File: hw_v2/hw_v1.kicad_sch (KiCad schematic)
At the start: 55 parts, among them J16 47352-1001, J8 USB_B, J9 Tag connect, SW2 SW_Push, U13 STM32F407VGTx, U14 TJA1051T-3, U15 25Q16, U16 REF3033, U17 SRV05-4, Y1 32.768kHz, Y2 25MHz

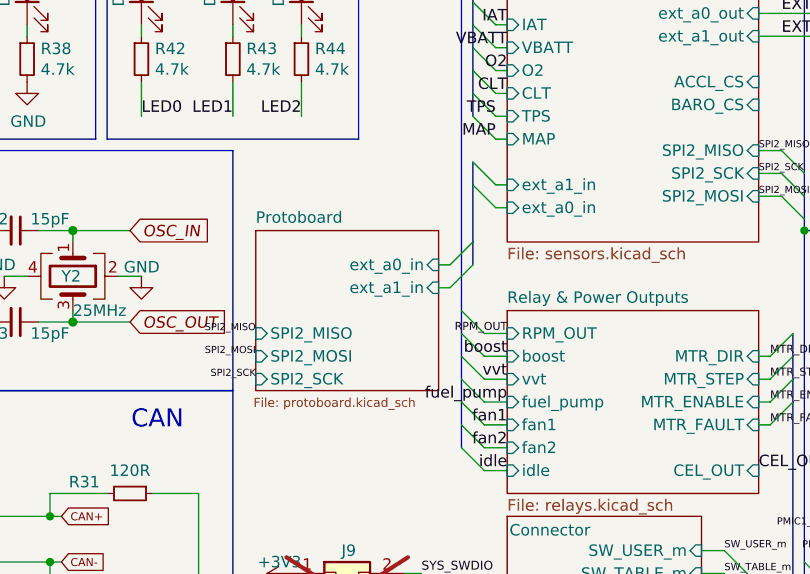
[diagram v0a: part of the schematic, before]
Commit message: wip v7
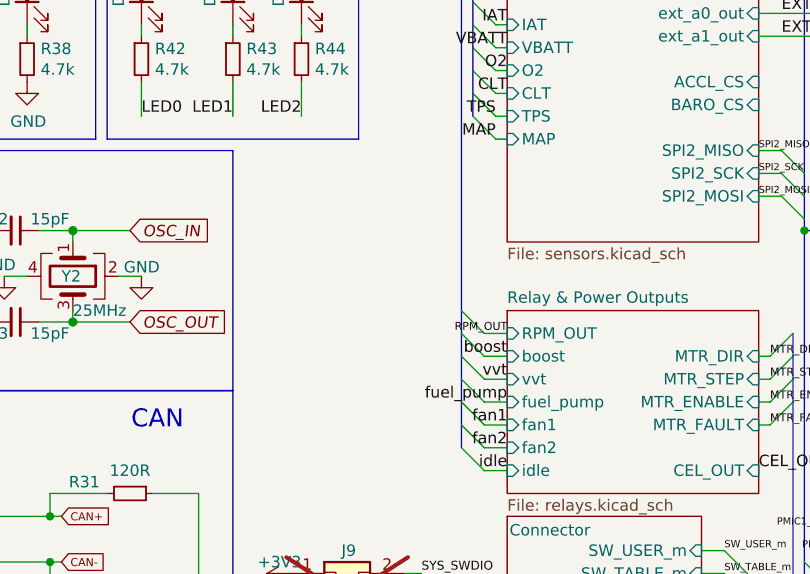
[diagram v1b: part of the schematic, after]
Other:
- removed sheet Protoboard
- sheet Sensors ports: added none; removed ext_a0_in, ext_a1_in
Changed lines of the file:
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@@
 	)
 	(bus_entry
-		(at 199.39 116.84)
-		(size 2.54 -2.54)
-		(stroke
-			(width 0)
-			(type default)
-		)
-	)
-	(bus_entry
 		(at 278.13 91.44)
 		(size 2.54 -2.54)
@@
 	)
 	(bus_entry
-		(at 201.93 105.41)
-		(size 2.54 2.54)
-		(stroke
-			(width 0)
-			(type default)
-		)
-	)
-	(bus_entry
 		(at 201.93 87.63)
 		(size 2.54 2.54)
@@
 	)
 	(bus_entry
-		(at 201.93 102.87)
-		(size 2.54 2.54)
-		(stroke
-			(width 0)
-			(type default)
-		)
-	)
-	(bus_entry
 		(at 88.9 66.04)
 		(size 2.54 2.54)
@@
 	)
 	(bus_entry
-		(at 199.39 114.3)
-		(size 2.54 -2.54)
-		(stroke
-			(width 0)
-			(type default)
-		)
-	)
-	(bus_entry
 		(at 276.86 154.94)
 		(size 2.54 -2.54)
@@
 	(wire
 		(pts
-			(xy 204.47 105.41) (xy 205.74 105.41)
-		)
-		(stroke
-			(width 0)
-			(type default)
-		)
-	)
-	(wire
-		(pts
 			(xy 81.28 124.46) (xy 95.25 124.46)
 		)
@@
 		)
 	)
-	(bus
-		(pts
-			(xy 201.93 102.87) (xy 201.93 105.41)
-		)
-		(stroke
-			(width 0)
-			(type default)
-		)
-	)
 	(wire
 		(pts
@@
 	(wire
 		(pts
-			(xy 198.12 116.84) (xy 199.39 116.84)
-		)
-		(stroke
-			(width 0)
-			(type default)
-		)
-	)
-	(wire
-		(pts
 			(xy 161.29 139.7) (xy 154.94 139.7)
 		)
@@
 		)
 	)
-	(wire
-		(pts
-			(xy 204.47 107.95) (xy 205.74 107.95)
-		)
-		(stroke
-			(width 0)
-			(type default)
-		)
-	)
 	(bus
 		(pts
@@
 	(wire
 		(pts
-			(xy 198.12 114.3) (xy 199.39 114.3)
-		)
-		(stroke
-			(width 0)
-			(type default)
-		)
-	)
-	(wire
-		(pts
 			(xy 55.88 38.1) (xy 55.88 40.64)
 		)
@@
 		)
 	)
-	(bus
-		(pts
-			(xy 201.93 111.76) (xy 201.93 114.3)
-		)
-		(stroke
-			(width 0)
-			(type default)
-		)
-	)
 	(wire
 		(pts
@@
 		)
 	)
-	(bus
-		(pts
-			(xy 201.93 105.41) (xy 201.93 111.76)
-		)
-		(stroke
-			(width 0)
-			(type default)
-		)
-	)
 	(wire
 		(pts
@@
 	)
 	(label "SPI2_MOSI"
-		(at 177.8 124.46 180)
-		(fields_autoplaced yes)
-		(effects
-			(font
-				(size 0.7874 0.7874)
-			)
-			(justify right bottom)
-		)
-	)
-	(label "SPI2_MOSI"
 		(at 83.82 129.54 0)
 		(fields_autoplaced yes)
@@
 		)
 	)
-	(label "SPI2_MISO"
-		(at 177.8 121.92 180)
-		(fields_autoplaced yes)
-		(effects
-			(font
-				(size 0.7874 0.7874)
-			)
-			(justify right bottom)
-		)
-	)
 	(label "CEL_OUT"
 		(at 83.82 134.62 0)
@@
 		)
 	)
-	(label "SPI2_SCK"
-		(at 177.8 127 180)
-		(fields_autoplaced yes)
-		(effects
-			(font
-				(size 0.7874 0.7874)
-			)
-			(justify right bottom)
-		)
-	)
 	(label "LED2"
 		(at 182.88 97.79 180)
@@
 	)
 	(sheet
-		(at 177.8 110.49)
-		(size 20.32 17.78)
-		(stroke
-			(width 0.1524)
-			(type solid)
-		)
-		(fill
-			(color 0 0 0 0.0000)
-		)
-		(property "Sheetname" "Protoboard"
-			(at 177.8 109.7784 0)
-			(effects
-				(font
-					(size 1.27 1.27)
-				)
-				(justify left bottom)
-			)
-		)
-		(property "Sheetfile" "protoboard.kicad_sch"
-			(at 177.546 129.032 0)
-			(effects
-				(font
-					(size 1 1)
-				)
-				(justify left top)
-			)
-		)
-		(pin "ext_a0_in" input
-			(at 198.12 114.3 0)
-			(effects
-				(font
-					(size 1.27 1.27)
-				)
-				(justify right)
-			)
-		)
-		(pin "ext_a1_in" input
-			(at 198.12 116.84 0)
-			(effects
-				(font
-					(size 1.27 1.27)
-				)
-				(justify right)
-			)
-		)
-		(pin "SPI2_MISO" input
-			(at 177.8 121.92 180)
-			(effects
-				(font
-					(size 1.27 1.27)
-				)
-				(justify left)
-			)
-		)
-		(pin "SPI2_MOSI" input
-			(at 177.8 124.46 180)
-			(effects
-				(font
-					(size 1.27 1.27)
-				)
-				(justify left)
-			)
-		)
-		(pin "SPI2_SCK" input
-			(at 177.8 127 180)
-			(effects
-				(font
-					(size 1.27 1.27)
-				)
-				(justify left)
-			)
-		)
-		(instances
-			(project "hw_v1"
-				(path "/b3feb07e-be80-40e1-bd13-6cd54c2f8b0c"
-					(page "7")
-				)
-			)
-		)
-	)
-	(sheet
 		(at 246.38 119.38)
 		(size 27.94 15.24)
@@
 			)
 		)
-		(pin "ext_a0_in" input
-			(at 205.74 107.95 180)
-			(effects
-				(font
-					(size 1.27 1.27)
-				)
-				(justify left)
-			)
-		)
 		(pin "ext_a1_out" input
 			(at 233.68 88.9 0)
@@
 			)
 		)
-		(pin "ext_a1_in" input
-			(at 205.74 105.41 180)
-			(effects
-				(font
-					(size 1.27 1.27)
-				)
-				(justify left)
-			)
-		)

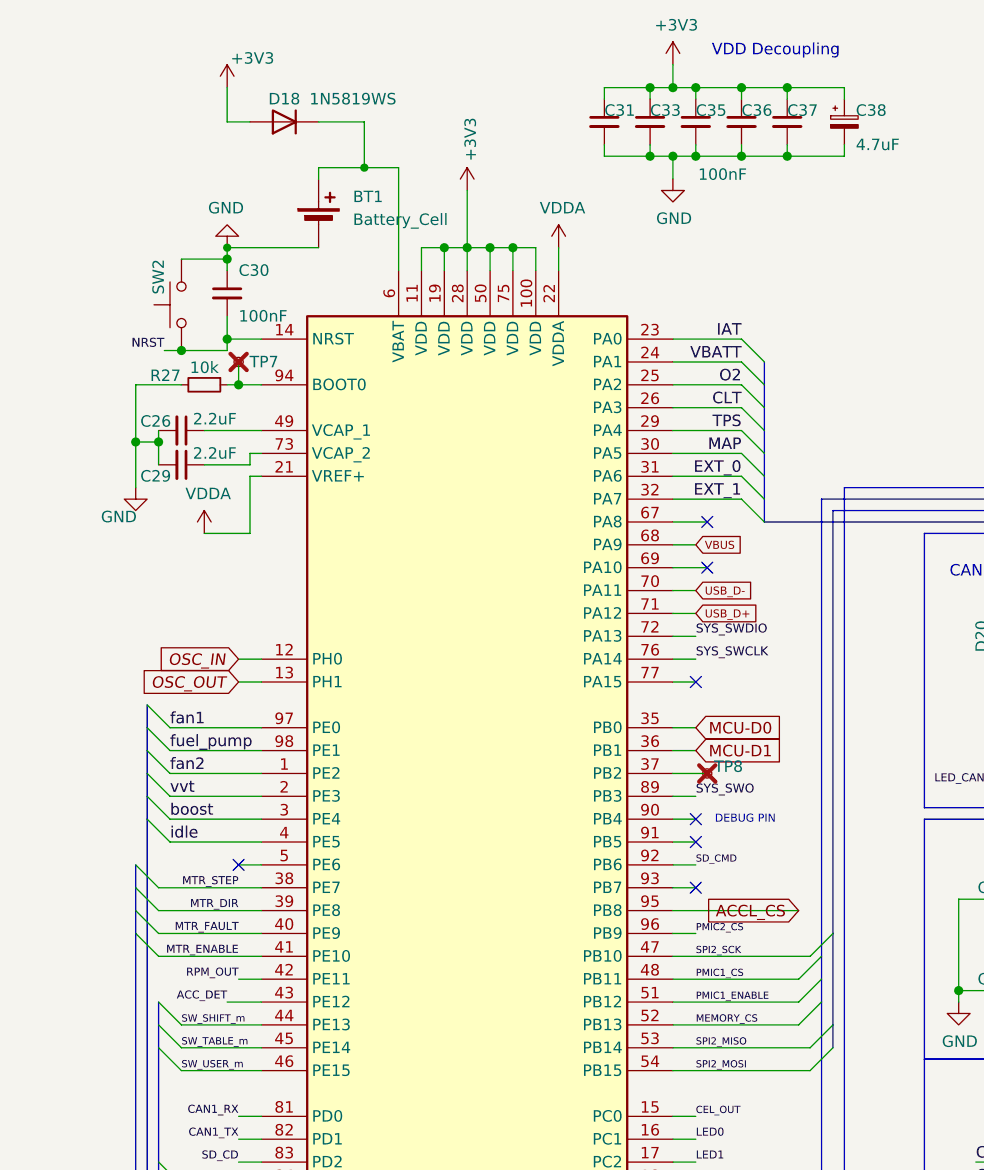
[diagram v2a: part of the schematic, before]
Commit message: hw v2
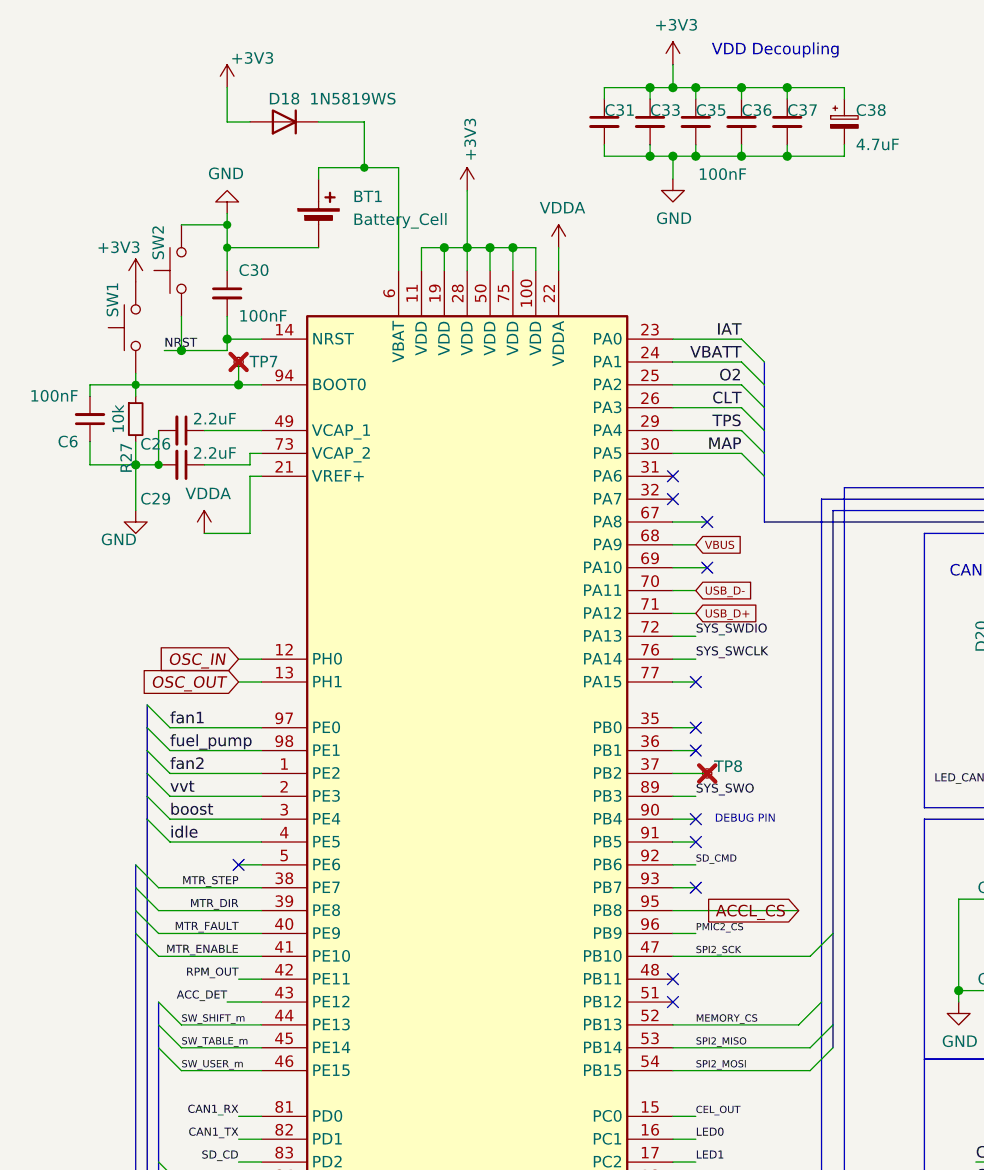
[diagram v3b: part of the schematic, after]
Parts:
- added C6: 100nF, Capacitor_SMD:C_0805_2012Metric, symbol Device:C_Small
- added SW1: SW_Push, Button_Switch_SMD:SW_SPST_CK_RS282G05A3, symbol Switch:SW_Push
- SW2: footprint Button_Switch_SMD:SW_SPST_TL3342 -> Button_Switch_SMD:SW_SPST_CK_RS282G05A3
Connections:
- net +3V3: now also SW1.2
- net EXT_0: no longer U13.31 (PA6)
- net EXT_1: no longer U13.32 (PA7)
- net GND: now also C6.1
- net PMIC1_CS: no longer U13.48 (PB11)
- net PMIC1_ENABLE: no longer U13.51 (PB12)
- net at R27.1, TP7.1, U13.94 (BOOT0): now also C6.2, SW1.1
- net MCU-D0: no longer names the net of U13.35 (PB0)
- net MCU-D1: no longer names the net of U13.36 (PB1)
- no-connect marks 10 -> 16
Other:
- moved on the sheet: R27, SW2
